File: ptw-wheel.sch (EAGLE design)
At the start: 3 parts

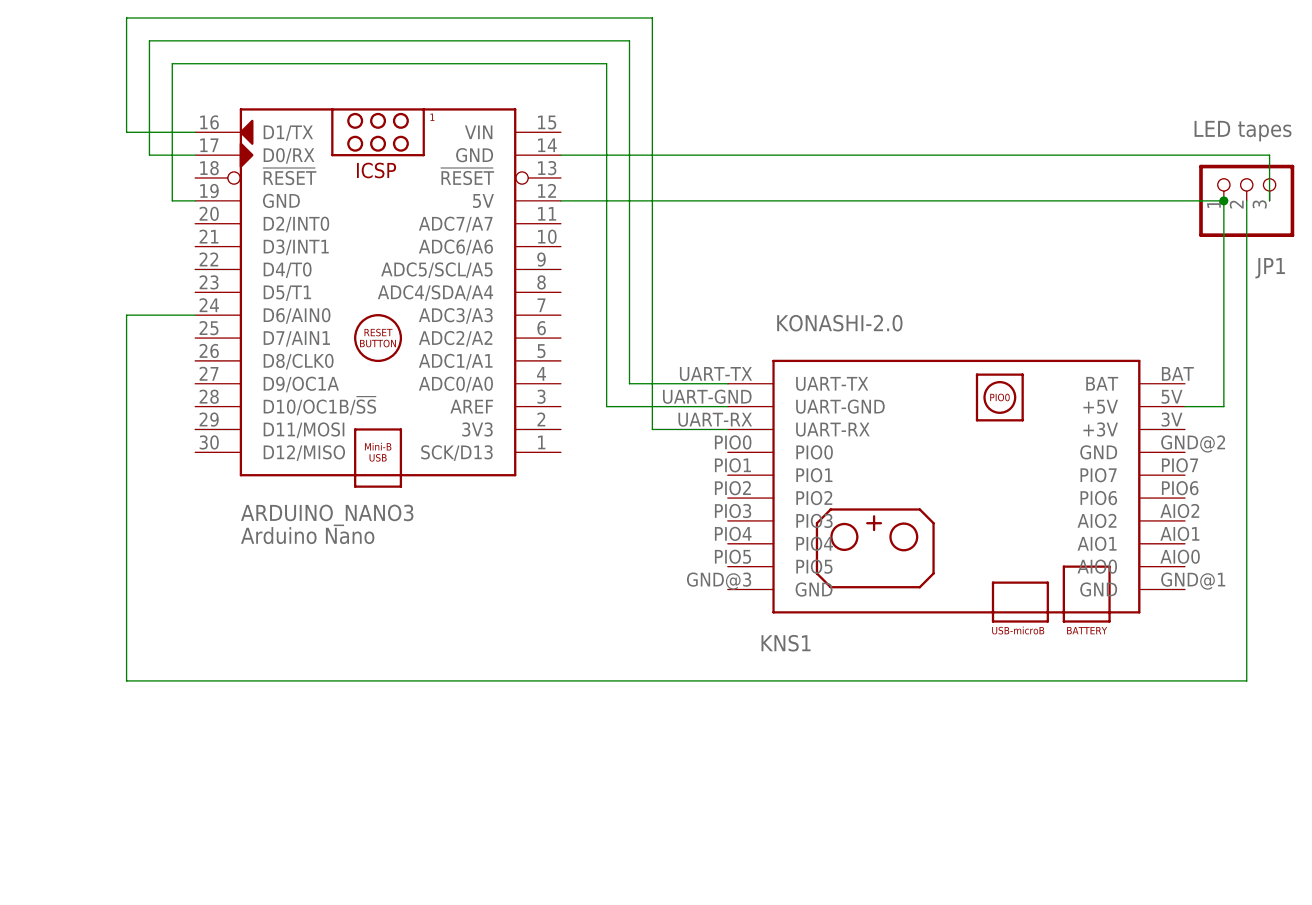
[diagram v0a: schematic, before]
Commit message: Create board data
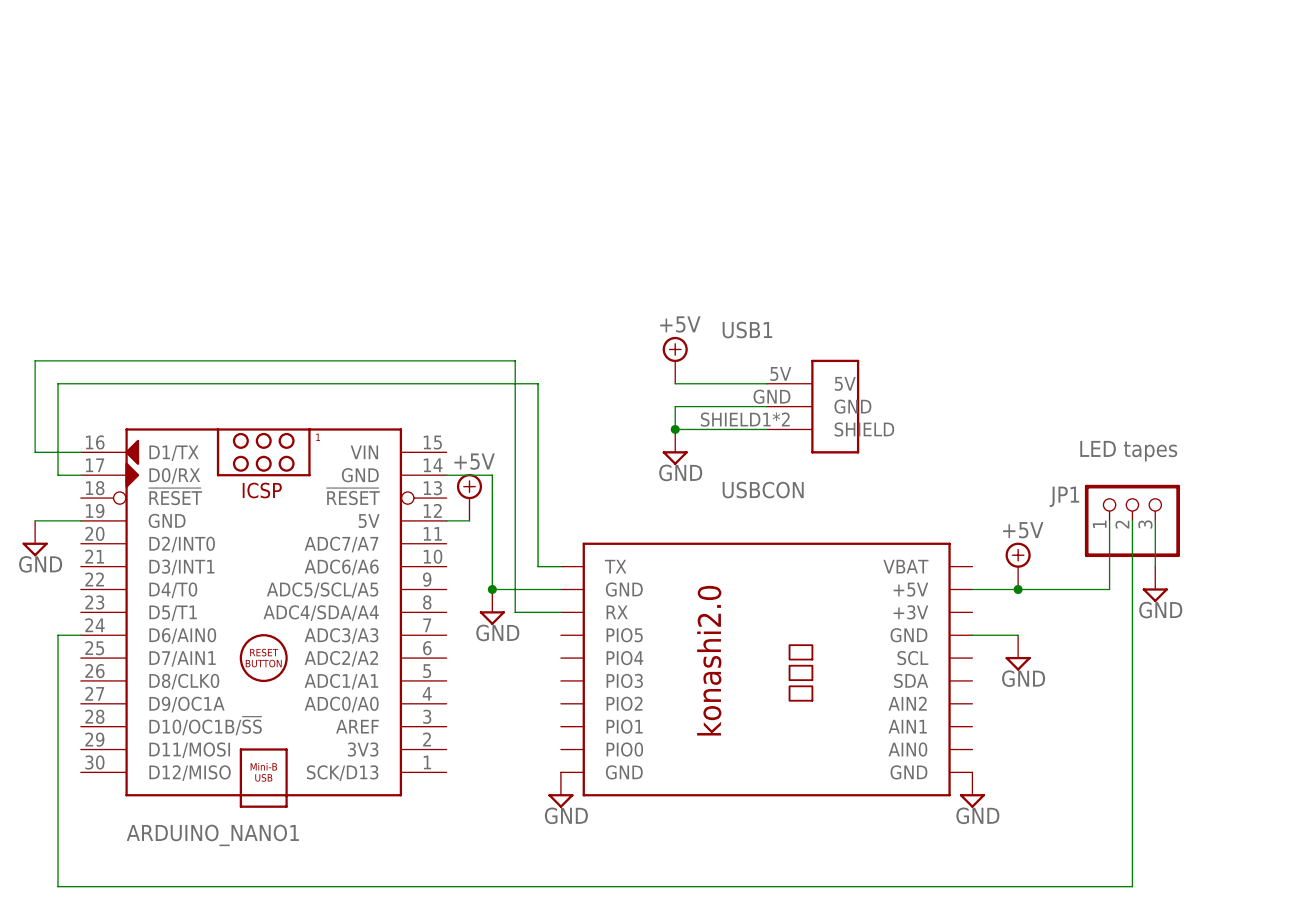
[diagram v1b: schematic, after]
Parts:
- removed ARDUINO_NANO3: Arduino Nano, ArduinoNanoV30:ARDUINO_NANO
- removed KNS1: KONASHI-2.0, konashi-2.0:KONASHI-2.0
- added ARDUINO_NANO1: (no value), arduinoNanoV30-withoud_drill_hole:ARDUINO_NANO
- added U$1: KONASHI2.0, konashiv2-withoud_drill_hole:KONASHI2.0
- added USB1: USBCON, usbcon:USBCON
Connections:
- removed net N$2: ARDUINO_NANO3.GND@2, JP1.3
- removed net N$6: ARDUINO_NANO3.GND@1, KNS1.UART-GND
- new net +5V: ARDUINO_NANO1.5V, JP1.1, U$1.+5V, USB1.5V
- new net GND: ARDUINO_NANO1.GND@1, JP1.3, U$1.GND, U$1.GND@1, U$1.GND@2, USB1.GND, USB1.SHIELD
- net N$1: now also ARDUINO_NANO1.GND@2, U$1.GND@3; no longer ARDUINO_NANO3.5V, JP1.1, KNS1.+5V
- net N$3: now also ARDUINO_NANO1.D6/AIN0; no longer ARDUINO_NANO3.D6/AIN0
- net N$4: now also ARDUINO_NANO1.D0/RX, U$1.TX; no longer ARDUINO_NANO3.D0/RX, KNS1.UART-TX
- net N$5: now also ARDUINO_NANO1.D1/TX, U$1.RX; no longer ARDUINO_NANO3.D1/TX, KNS1.UART-RX
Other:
- moved on the sheet: JP1
